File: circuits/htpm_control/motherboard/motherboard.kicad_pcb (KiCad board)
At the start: 2 copper layers, 51 parts, among them J3 Conn_01x40_Socket, J5 Connector_Modcore, J6 Motor_Power, J7 Connector_Display, J8 Connector_Motor_Driver, U1 74HC165, U2 74HC165, U3 74HC165, U4 74HC165, U5 74HC595, U6 74HC595, U7 L7805

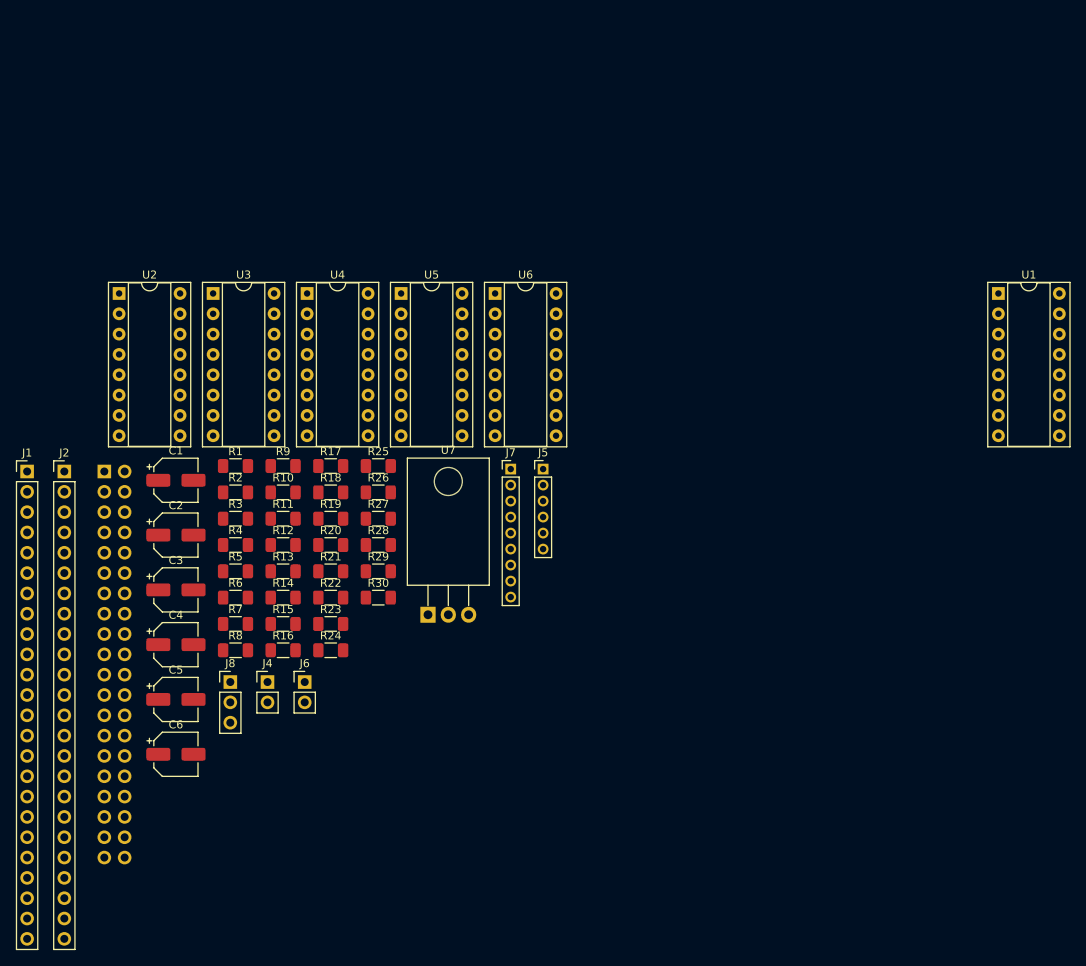
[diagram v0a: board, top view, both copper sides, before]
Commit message: Created HTPm CONTROL Motherboard PCB.
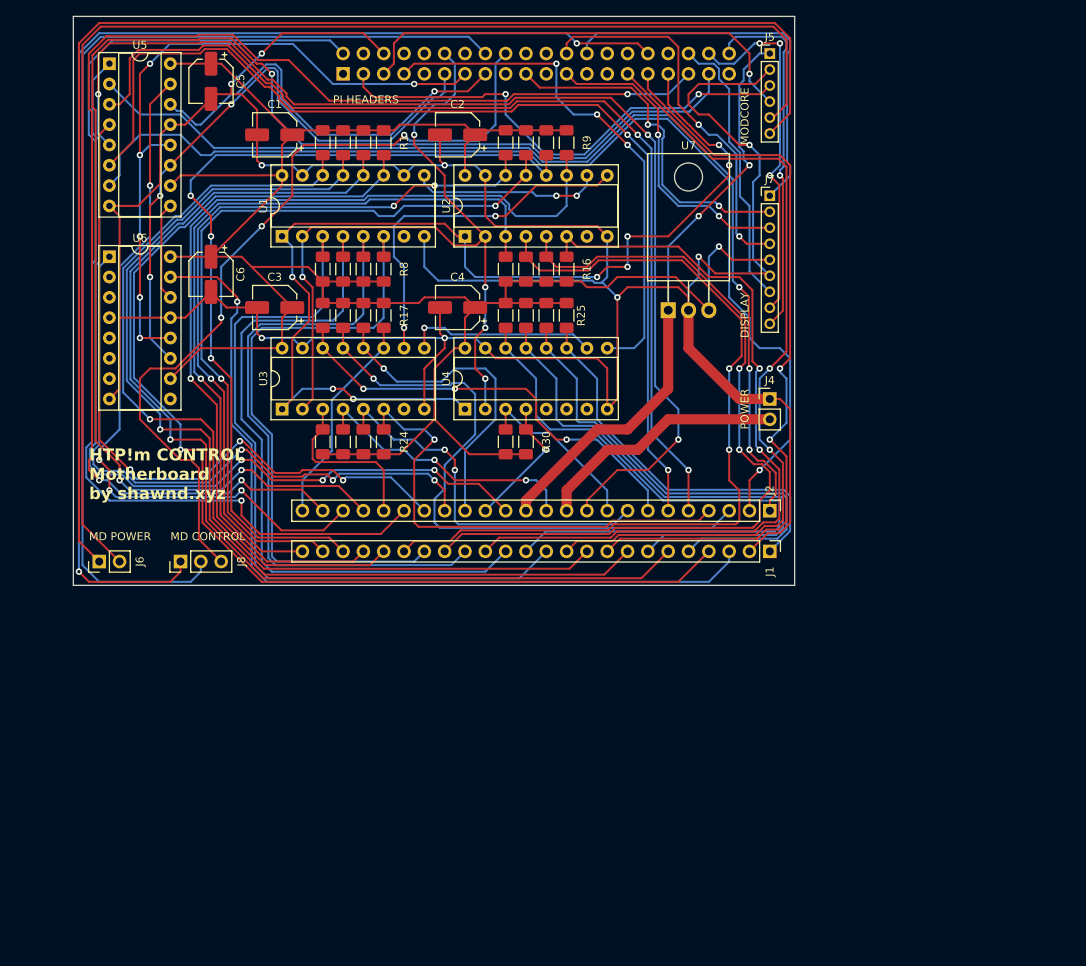
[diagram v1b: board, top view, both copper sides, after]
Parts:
- R1, R10, R11, R12, R13, R14, R15, R16, R17, R18, R19, R2, R20, R21, R22, R23, R24, R25, R26, R27, R28, R29, R3, R30, R4, R5, R6, R7, R8, R9: value 10kΩ -> 4.7kΩ
- moved J1 93.4 mm to (141.6, 90.8), turned to -90 degrees
- moved U1 89.8 mm to (80.6, 51.4), turned to 90 degrees
- moved J2 88.3 mm to (141.6, 85.7), turned to -90 degrees
- moved C5 77.4 mm to (71.8, 32.0), turned to -90 degrees
- moved J4 72.1 mm to (141.6, 71.8)
- moved C2 61.2 mm to (102.6, 38.7), turned to 180 degrees
- moved C6 60.2 mm to (71.8, 56.2), turned to -90 degrees
- moved R16 59.4 mm to (116.2, 55.5), turned to 90 degrees
- moved J5 59.2 mm to (141.6, 28.6)
- moved J3 58.0 mm to (88.3, 31.1), turned to -90 degrees
- moved R12 57.5 mm to (108.6, 39.7), turned to -90 degrees
- moved R11 55.9 mm to (111.1, 39.7), turned to -90 degrees
- moved R15 55.2 mm to (113.7, 55.5), turned to 90 degrees
- moved C4 54.9 mm to (102.6, 60.3), turned to 180 degrees
- moved R10 54.7 mm to (113.7, 39.7), turned to -90 degrees
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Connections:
- J1 pad 2: Net-(J1-GND) -> GND
- J3 pad 6: Net-(J1-GND) -> GND
- J4 pad 1: Net-(J1-GND) -> GND
- J5 pad 2: Net-(J1-GND) -> GND
- J7 pad 6: Net-(J1-GND) -> GND
- U7 pad 2: Net-(J1-GND) -> GND
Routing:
- net GND: track 0.00 -> 389.9 mm, vias 0 -> 9
- net Net-(J7-5V): track 0.00 -> 276.5 mm, vias 0 -> 1
- net Net-(J2-TIME_SET_DT): track 0.00 -> 181.4 mm, vias 0 -> 3
- net Net-(J5-VA): track 0.00 -> 169.5 mm
- net Net-(J5-VB): track 0.00 -> 167.0 mm
- net Net-(J2-TIME_SET_CLK): track 0.00 -> 165.8 mm, vias 0 -> 3
- net Net-(J3-GPIO12(PWM0)): track 0.00 -> 153.0 mm, vias 0 -> 2
- net Net-(J1-BIT_0): track 0.00 -> 143.0 mm, vias 0 -> 1
- net Net-(J2-11_LED): track 0.00 -> 142.5 mm, vias 0 -> 3
- net Net-(J2-13_LED): track 0.00 -> 137.2 mm, vias 0 -> 1
- net Net-(J1-BIT_1): track 0.00 -> 136.1 mm, vias 0 -> 1
- net Net-(J3-GPIO13(PWM1)): track 0.00 -> 135.0 mm, vias 0 -> 8
- net Net-(J3-GPIO23): track 0.00 -> 133.4 mm
- net Net-(J2-02_LED): track 0.00 -> 132.1 mm, vias 0 -> 3
- net Net-(J2-12_LED): track 0.00 -> 131.2 mm, vias 0 -> 2
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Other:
- board outline added: 90.2 x 71.1 mm
- board text added: "DISPLAY"
- board text added: "HTP!m CONTROL Motherboard by shawnd.xyz"
- board text added: "JLCJLCJLCJLC"
- board text added: "MD CONTROL"
- board text added: "MD POWER"
- board text added: "MODCORE"
- board text added: "PI HEADERS"
- board text added: "POWER"
